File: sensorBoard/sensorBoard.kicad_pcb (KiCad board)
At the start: 4 copper layers, 203.9 x 100 mm, 164 parts, among them J10 Conn_01x07, J11 Conn_01x03, J12 Conn_01x02, J13 Conn_01x04, J14 Conn_01x05, J15 Conn_01x02, J16 Conn_01x02, J17 Conn_01x04, J18 Conn_01x07, J19 Conn_01x03, J20 Conn_01x02, J21 Conn_01x04, J22 Conn_01x05, J23 Conn_01x02, J24 Conn_01x02, J9 Conn_01x04, K5 G2RL-1-H, K6 G2RL-1-H, Q10 2N7002, Q11 2SC4213, Q12 NTD3055, Q19 2SC4213, Q2 2N7002, Q20 NTD3055, Q21 2N7002, Q22 2N7002, Q23 BSC440N10NS3G, Q24 BSC440N10NS3G, Q25 BSC440N10NS3G, Q26 BSC440N10NS3G, U12 MCP2551-I-SN, U17 LD1117S33TR_SOT223, U20 BTS50080-1TEA, U21 LM75C, U23 STM32L476RGTx, U32 BTS50080-1TEA, U33 LM75C, U35 STM32L476RGTx, U36 4011, U38 4011, U39 4011, U40 4011, U42 4N25, U43 4N25, U7 LD1117S33TR_SOT223, U9 MCP2551-I-SN, Y2 8MHz, Y3 8MHz

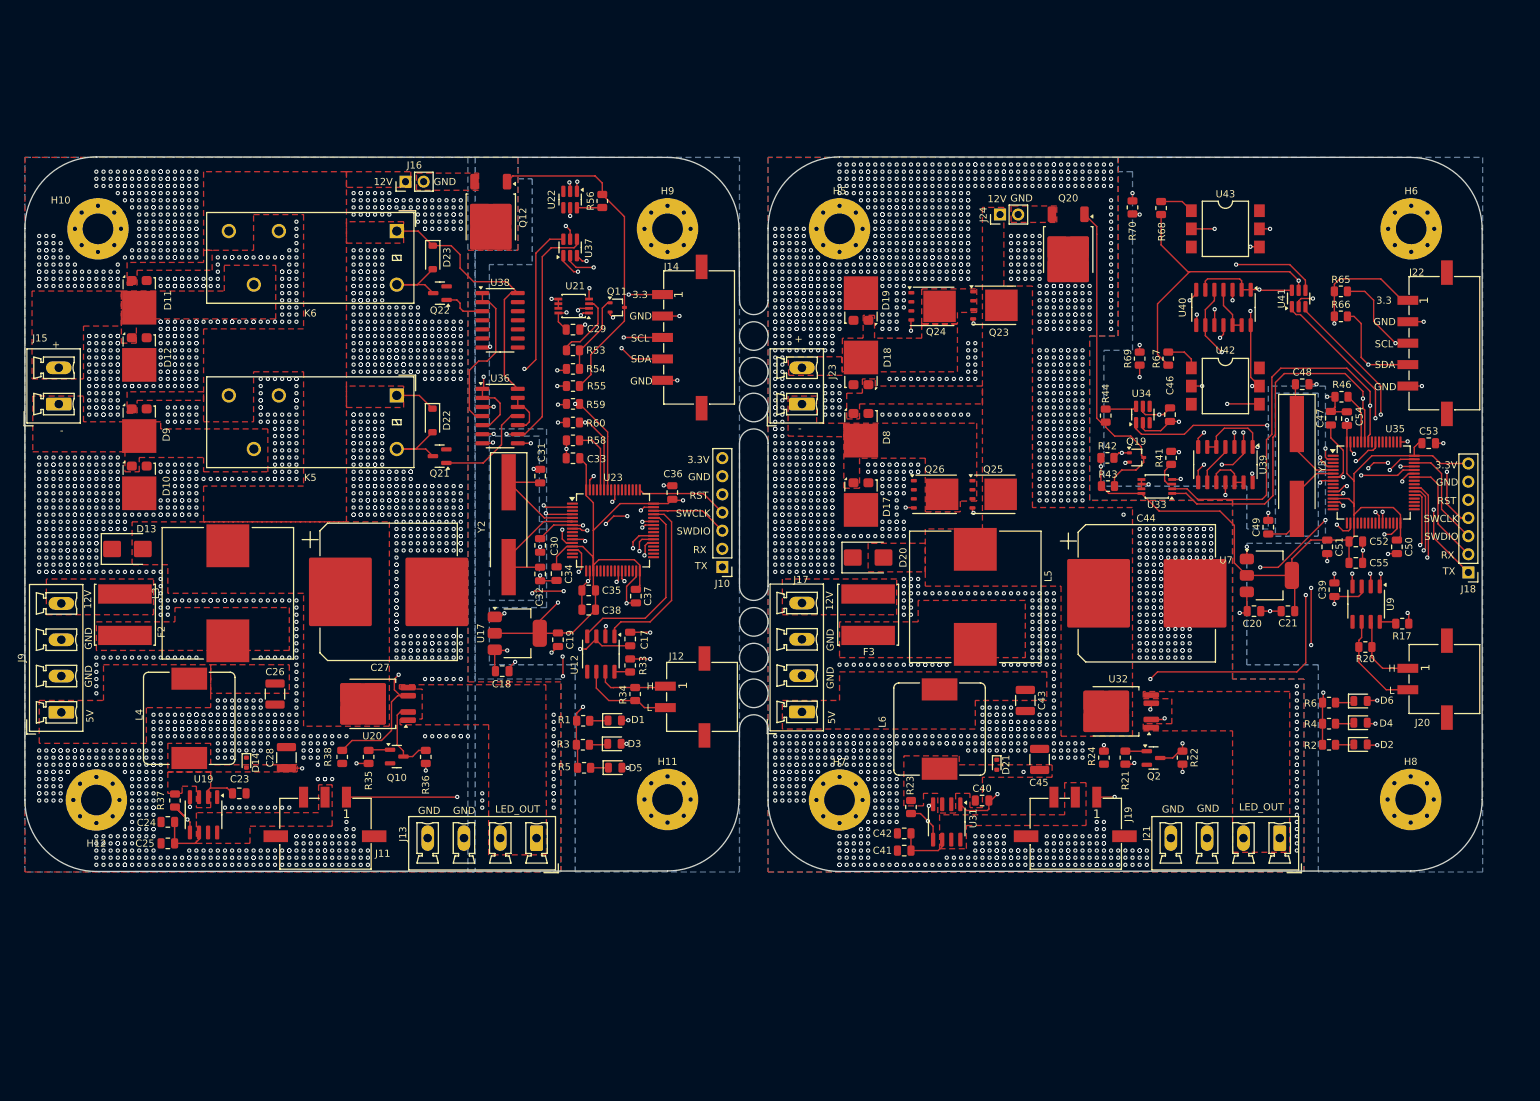
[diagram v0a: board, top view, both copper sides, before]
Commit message: aktualisierte Platine mit verschiedenen Stecker
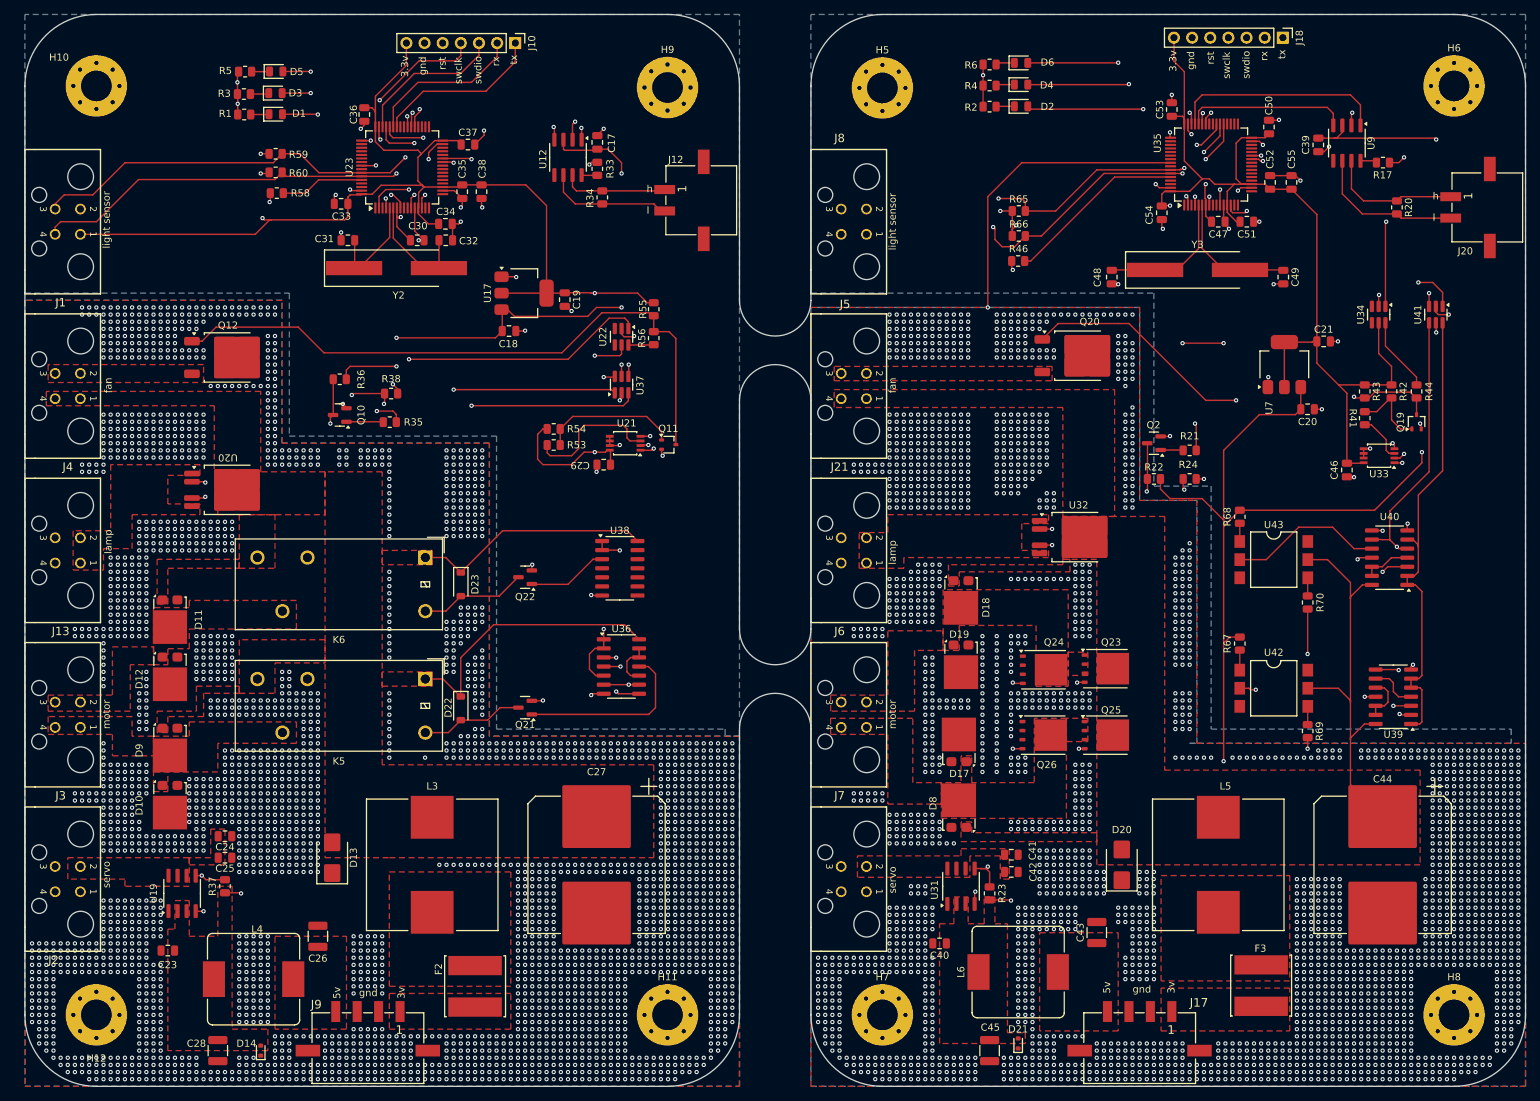
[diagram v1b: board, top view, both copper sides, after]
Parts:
- removed J11, J19: Conn_01x03, heder box:662103145021
- removed J14, J22: Conn_01x05, heder box:662105145021
- removed J15, J23: Conn_01x02, Connector_Phoenix_MC_HighVoltage:PhoenixContact_MCV_1,5_2-G-5.08_1x02_P5.08mm_Vertical
- removed J16, J24: Conn_01x02, Connector_PinHeader_2.54mm:PinHeader_1x02_P2.54mm_Vertical
- added J1: Conn_01x04, 6432101004xx:643210100404, F.Cu at (36.0, 49.0)
- added J2: Conn_01x04, 6432101004xx:643210100404, F.Cu at (36.0, 141.0)
- added J3: Conn_01x04, 6432101004xx:643210100404, F.Cu at (36.0, 118.0)
- added J4: Conn_01x04, 6432101004xx:643210100404, F.Cu at (36.0, 72.0)
- added J5: Conn_01x04, 6432101004xx:643210100404, F.Cu at (146.0, 72.0)
- added J6: Conn_01x04, 6432101004xx:643210100404, F.Cu at (146.0, 118.0)
- added J7: Conn_01x04, 6432101004xx:643210100404, F.Cu at (146.0, 141.0)
- added J8: Conn_01x04, 6432101004xx:643210100404, F.Cu at (146.0, 49.0)
- J13, J21: footprint Connector_Phoenix_MC_HighVoltage:PhoenixContact_MCV_1,5_4-G-5.08_1x04_P5.08mm_Vertical -> 6432101004xx:643210100404
- J17, J9: footprint Connector_Phoenix_MC_HighVoltage:PhoenixContact_MCV_1,5_4-G-5.08_1x04_P5.08mm_Vertical -> heder box:662104145021
- moved D5 108.4 mm to (65.2, 28.0)
- moved R5 108.4 mm to (60.8, 28.0)
- moved D3 102.7 mm to (65.1, 31.0)
- moved R3 102.7 mm to (60.7, 31.1)
- moved D2 101.1 mm to (169.4, 32.9)
- moved D4 101.1 mm to (169.4, 29.8)
- moved D6 101.1 mm to (169.4, 26.8)
- moved R2 101.1 mm to (165.0, 32.9)
- moved R4 101.1 mm to (165.0, 29.9)
- moved R6 101.1 mm to (165.0, 27.0)
- moved D1 97.2 mm to (65.1, 34.0)
- moved R1 97.2 mm to (60.7, 34.0)
- moved J18 79.2 mm to (206.0, 23.2), turned to -90 degrees
- moved J10 78.8 mm to (98.6, 24.0), turned to -90 degrees
- moved J13 77.0 mm to (36.0, 95.0), turned to -90 degrees
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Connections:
- J17 pad 1: /Platine2/Protection2/5V_IN -> /Platine2/Protection2/12V_IN
- J17 pad 4: /Platine2/Protection2/12V_IN -> /Platine2/Protection2/5V_IN
- J18 pad 1: /Platine2/microcontroller2/UART_RX -> /Platine2/microcontroller2/UART_TX
- J18 pad 2: /Platine2/microcontroller2/UART_TX -> /Platine2/microcontroller2/UART_RX
- J9 pad 1: /Platine1/Protection1/5V_IN -> /Platine1/Protection1/12V_IN
- J9 pad 4: /Platine1/Protection1/12V_IN -> /Platine1/Protection1/5V_IN
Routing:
- net +5V: track 307.2 -> 407.7 mm, vias 10 -> 11
- net /Platine1/SERVO_PWM: track 59.8 -> 153.7 mm, vias 2 -> 1
- net /Platine1/I2C_SDA: track 42.1 -> 133.7 mm, vias 3 -> 2
- net /Platine1/I2C_SCL: track 42.6 -> 129.7 mm, vias 3 -> 2
- net /Platine2/SERVO_PWM: track 67.7 -> 135.6 mm, vias 2 -> 3
- net +3.3V: track 330.3 -> 394.1 mm, vias 13 -> 9
- net /Platine2/I2C_SDA: track 71.3 -> 126.7 mm, vias 2 -> 3
- net /Platine2/I2C_SCL: track 77.1 -> 124.5 mm, vias 2 -> 3
- net /Platine1/Commutation1-1/SERVO_EN: track 83.7 -> 130.2 mm, vias 4 -> 2
- net Net-(Q11-C): track 46.4 -> 90.0 mm
- net /Platine2/Commutation2-2/SERVO_EN: track 96.8 -> 131.3 mm
- net +12V: track 101.7 -> 130.1 mm, vias 5 -> 0
- net GND: track 140.5 -> 116.1 mm, vias 4023 -> 5395
- net /Platine1/Commutation1-1/OVER_CURR_SERVO: track 109.8 -> 133.5 mm
- net /Platine1/LED_EN: track 58.9 -> 35.6 mm
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- added copper zone on In2.Cu, net GND
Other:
- board size 203.9 x 100 mm -> 210 x 150 mm
- board text added: "3.3v"
- board text added: "3v"
- board text added: "5v"
- board text added: "fan"
- board text added: "gnd"
- board text added: "h"
- board text added: "l"
- board text added: "lamp"
- board text added: "light sensor"
- board text added: "motor"
- board text added: "rst"
- board text added: "rx"
- board text added: "servo"
- board text added: "swclk"
- board text added: "swdio"
- board text added: "tx"
- board text removed: "+"
- board text removed: "-"
- board text removed: "12V"
- board text removed: "3.3"
- board text removed: "3.3V"
- board text removed: "5V"
- board text removed: "GND"
- board text removed: "H"
- board text removed: "L"
- board text removed: "LED_OUT"
- board text removed: "RST"
- board text removed: "RX"
- board text removed: "SCL"
- board text removed: "SDA"
- board text removed: "SWCLK"
- board text removed: "SWDIO"
- board text removed: "TX"
